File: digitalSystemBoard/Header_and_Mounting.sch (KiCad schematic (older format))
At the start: 16 parts, among them J10 Conn_02x03_Odd_Even, J11 Conn_02x03_Odd_Even, J12 Conn_02x03_Odd_Even, J3 Conn_02x04_Odd_Even, J4 Conn_02x04_Odd_Even, J5 Conn_02x08_Odd_Even, J6 Conn_02x07_Odd_Even, J7 Conn_02x07_Odd_Even, J8 Conn_02x08_Odd_Even, J9 Conn_02x03_Odd_Even

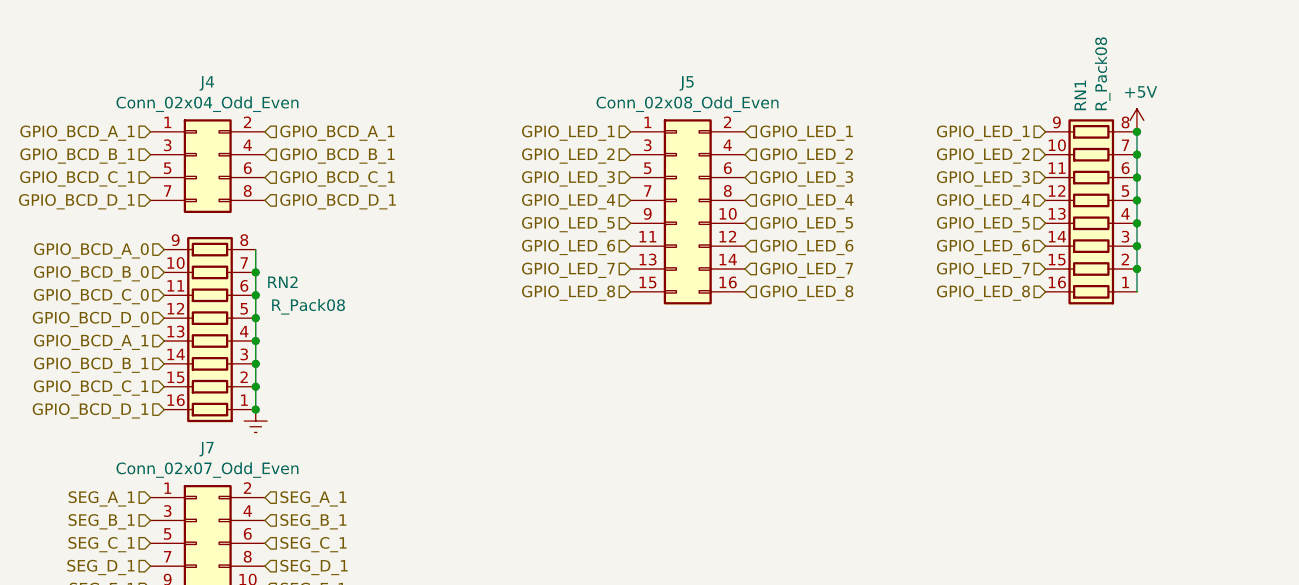
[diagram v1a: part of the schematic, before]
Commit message: Replace R array by 16 single R
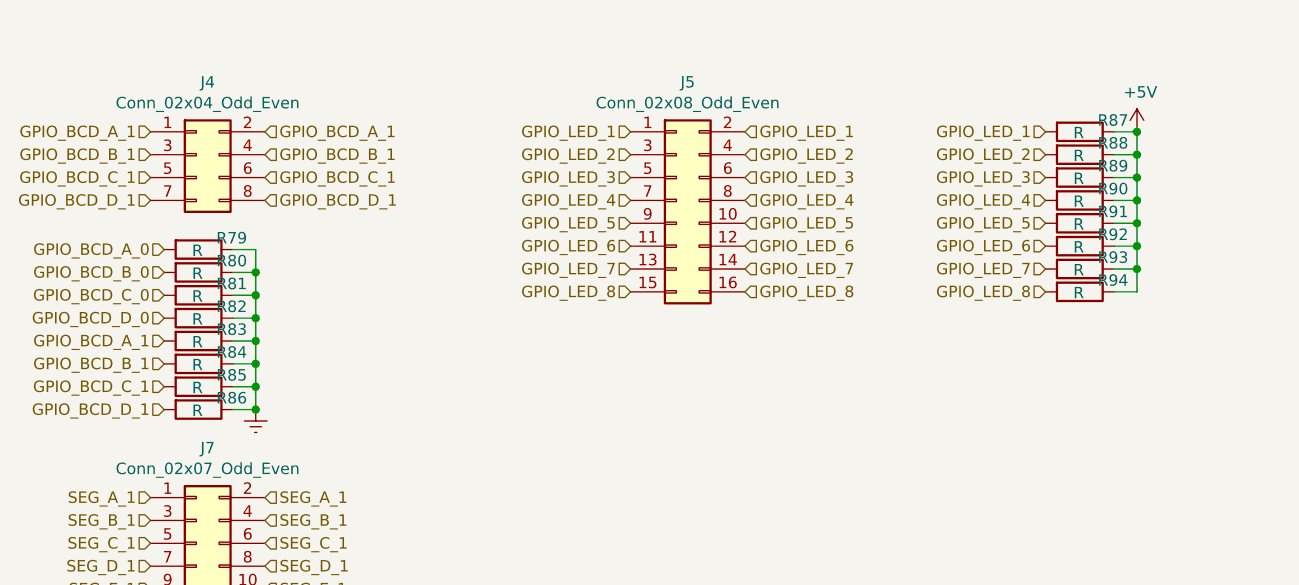
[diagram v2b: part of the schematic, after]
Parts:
- removed RN1, RN2: R_Pack08, digitalSystemBoard:Resistor Bar 06030 8P4R, symbol Device:R_Pack08
- added R79, R80, R81, R82, R83, R84, R85, R86, R87, R88, R89, R90, R91, R92, R93, R94: R, Resistor_SMD:R_0603_1608Metric, symbol Device:R
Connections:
- net +5V: now also R87.1, R88.1, R89.1, R90.1, R91.1, R92.1, R93.1, R94.1
- net Earth: now also R79.1, R80.1, R81.1, R82.1, R83.1, R84.1, R85.1, R86.1
- net GPIO_BCD_A_0: now also R79.2
- net GPIO_BCD_A_1: now also R83.2
- net GPIO_BCD_B_0: now also R80.2
- net GPIO_BCD_B_1: now also R84.2
- net GPIO_BCD_C_0: now also R81.2
- net GPIO_BCD_C_1: now also R85.2
- net GPIO_BCD_D_0: now also R82.2
- net GPIO_BCD_D_1: now also R86.2
- net GPIO_LED_1: now also R87.2
- net GPIO_LED_2: now also R88.2
- net GPIO_LED_3: now also R89.2
- net GPIO_LED_4: now also R90.2
- net GPIO_LED_5: now also R91.2
- net GPIO_LED_6: now also R92.2
- net GPIO_LED_7: now also R93.2
- net GPIO_LED_8: now also R94.2
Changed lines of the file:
@@
-$EndComp
-$Comp
-L Connector_Generic:Conn_02x04_Odd_Even J4
-U 1 1 5FC88FC0
-P 4000 2100
-F 0 "J4" H 4050 2417 50  0000 C CNN
-F 1 "Conn_02x04_Odd_Even" H 4050 2326 50  0000 C CNN
-F 2 "Connector_IDC:IDC-Header_2x04_P2.54mm_Vertical" H 4000 2100 50  0001 C CNN
-F 3 "~" H 4000 2100 50  0001 C CNN
-	1    4000 2100
-	1    0    0    -1
 $EndComp
 $Comp
@@
 SEG_A_1
 $Comp
-L Device:R_Pack08 RN1
-U 1 1 6033D84A
-P 7915 2300
-F 0 "RN1" H 8303 2346 50  0000 L CNN
-F 1 "R_Pack08" H 8303 2255 50  0000 L CNN
-F 2 "digitalSystemBoard:Resistor Bar 06030 8P4R" V 8390 2300 50  0001 C CNN
-F 3 "~" H 7915 2300 50  0001 C CNN
-	1    7915 2300
-	0    -1   -1   0
-$EndComp
-$Comp
-L Device:R_Pack08 RN2
-U 1 1 6033EE65
-P 4060 2815
-F 0 "RN2" V 4215 2425 50  0000 L CNN
-F 1 "R_Pack08" V 4115 2220 50  0000 L CNN
-F 2 "digitalSystemBoard:Resistor Bar 06030 8P4R" V 4535 2815 50  0001 C CNN
-F 3 "~" H 4060 2815 50  0001 C CNN
-	1    4060 2815
-	0    -1   -1   0
-$EndComp
-$Comp
 L power:+5V #PWR0101
 U 1 1 6049CAFD
@@
 	1    0    0    -1
 $EndComp
-Wire Wire Line
-	8115 2000 8115 2100
-Connection ~ 8115 2000
-Wire Wire Line
-	8115 2100 8115 2200
-Connection ~ 8115 2100
-Wire Wire Line
-	8115 2200 8115 2300
-Connection ~ 8115 2200
-Wire Wire Line
-	8115 2300 8115 2400
-Connection ~ 8115 2300
-Wire Wire Line
-	8115 2400 8115 2500
-Connection ~ 8115 2400
-Wire Wire Line
-	8115 2500 8115 2600
-Connection ~ 8115 2500
-Wire Wire Line
-	8115 2600 8115 2700
-Connection ~ 8115 2600
 Text HLabel 7715 2700 0    50   Input ~ 0
 GPIO_LED_8
@@
 Text HLabel 7715 2000 0    50   Input ~ 0
 GPIO_LED_1
-$Comp
-L power:Earth #PWR0102
-U 1 1 604ACAC7
-P 4260 3215
-F 0 "#PWR0102" H 4260 2965 50  0001 C CNN
-F 1 "Earth" H 4260 3065 50  0001 C CNN
-F 2 "" H 4260 3215 50  0001 C CNN
-F 3 "~" H 4260 3215 50  0001 C CNN
-	1    4260 3215
-	1    0    0    -1
-$EndComp
-Wire Wire Line
-	4260 2515 4260 2615
-Wire Wire Line
-	4260 2615 4260 2715
-Connection ~ 4260 2615
-Wire Wire Line
-	4260 2715 4260 2815
-Connection ~ 4260 2715
-Wire Wire Line
-	4260 2815 4260 2915
-Connection ~ 4260 2815
-Wire Wire Line
-	4260 2915 4260 3015
-Connection ~ 4260 2915
-Wire Wire Line
-	4260 3015 4260 3115
-Connection ~ 4260 3015
-Wire Wire Line
-	4260 3115 4260 3215
-Connection ~ 4260 3115
-Connection ~ 4260 3215
 Text HLabel 3860 2515 0    50   Input ~ 0
 GPIO_BCD_A_0
@@
 Text HLabel 3860 3215 0    50   Input ~ 0
 GPIO_BCD_D_1
+$Comp
+L Connector_Generic:Conn_02x04_Odd_Even J4
+U 1 1 5FC88FC0
+P 4000 2100
+F 0 "J4" H 4050 2417 50  0000 C CNN
+F 1 "Conn_02x04_Odd_Even" H 4050 2326 50  0000 C CNN
+F 2 "Connector_IDC:IDC-Header_2x04_P2.54mm_Vertical" H 4000 2100 50  0001 C CNN
+F 3 "~" H 4000 2100 50  0001 C CNN
+	1    4000 2100
+	1    0    0    -1
+$EndComp
+Connection ~ 4260 3215
+Wire Wire Line
+	4160 3215 4260 3215
+Wire Wire Line
+	4260 3115 4260 3215
+Connection ~ 4260 3115
+Wire Wire Line
+	4160 3115 4260 3115
+Wire Wire Line
+	4260 3015 4260 3115
+Connection ~ 4260 3015
+Wire Wire Line
+	4160 3015 4260 3015
+Wire Wire Line
+	4260 2915 4260 3015
+Connection ~ 4260 2915
+Wire Wire Line
+	4160 2915 4260 2915
+Wire Wire Line
+	4260 2815 4260 2915
+Connection ~ 4260 2815
+Wire Wire Line
+	4160 2815 4260 2815
+Wire Wire Line
+	4260 2715 4260 2815
+Connection ~ 4260 2715
+Wire Wire Line
+	4160 2715 4260 2715
+Wire Wire Line
+	4260 2615 4260 2715
+Connection ~ 4260 2615
+Wire Wire Line
+	4160 2615 4260 2615
+Wire Wire Line
+	4260 2515 4160 2515
+$Comp
+L Device:R R86
+U 1 1 60520B8F
+P 4010 3215
+F 0 "R86" V 3960 3360 50  0000 C CNN
+F 1 "R" V 4015 3210 50  0000 C CNN
+F 2 "Resistor_SMD:R_0603_1608Metric" V 3940 3215 50  0001 C CNN
+F 3 "~" H 4010 3215 50  0001 C CNN
+	1    4010 3215
+	0    1    1    0
+$EndComp
+$Comp
+L Device:R R85
+U 1 1 605206C3
+P 4010 3115
+F 0 "R85" V 3960 3260 50  0000 C CNN
+F 1 "R" V 4015 3110 50  0000 C CNN
+F 2 "Resistor_SMD:R_0603_1608Metric" V 3940 3115 50  0001 C CNN
+F 3 "~" H 4010 3115 50  0001 C CNN
+	1    4010 3115
+	0    1    1    0
+$EndComp
+$Comp
+L Device:R R84
+U 1 1 605202F2
+P 4010 3015
+F 0 "R84" V 3960 3160 50  0000 C CNN
+F 1 "R" V 4015 3010 50  0000 C CNN
+F 2 "Resistor_SMD:R_0603_1608Metric" V 3940 3015 50  0001 C CNN
+F 3 "~" H 4010 3015 50  0001 C CNN
+	1    4010 3015
+	0    1    1    0
+$EndComp
+$Comp
+L Device:R R83
+U 1 1 6051FA6A
+P 4010 2915
+F 0 "R83" V 3960 3060 50  0000 C CNN
+F 1 "R" V 4015 2910 50  0000 C CNN
+F 2 "Resistor_SMD:R_0603_1608Metric" V 3940 2915 50  0001 C CNN
+F 3 "~" H 4010 2915 50  0001 C CNN
+	1    4010 2915
+	0    1    1    0
+$EndComp
+$Comp
+L Device:R R82
+U 1 1 6051F3E2
+P 4010 2815
+F 0 "R82" V 3960 2960 50  0000 C CNN
+F 1 "R" V 4015 2810 50  0000 C CNN
+F 2 "Resistor_SMD:R_0603_1608Metric" V 3940 2815 50  0001 C CNN
+F 3 "~" H 4010 2815 50  0001 C CNN
+	1    4010 2815
+	0    1    1    0
+$EndComp
+$Comp
+L Device:R R81
+U 1 1 6051ECC9
+P 4010 2715
+F 0 "R81" V 3960 2860 50  0000 C CNN
+F 1 "R" V 4015 2710 50  0000 C CNN
+F 2 "Resistor_SMD:R_0603_1608Metric" V 3940 2715 50  0001 C CNN
+F 3 "~" H 4010 2715 50  0001 C CNN
+	1    4010 2715
+	0    1    1    0
+$EndComp
+$Comp
+L Device:R R80
+U 1 1 6051E775
+P 4010 2615
+F 0 "R80" V 3960 2760 50  0000 C CNN
+F 1 "R" V 4015 2610 50  0000 C CNN
+F 2 "Resistor_SMD:R_0603_1608Metric" V 3940 2615 50  0001 C CNN
+F 3 "~" H 4010 2615 50  0001 C CNN
+	1    4010 2615
+	0    1    1    0
+$EndComp
+$Comp
+L Device:R R79
+U 1 1 6051C220
+P 4010 2515
+F 0 "R79" V 3960 2660 50  0000 C CNN
+F 1 "R" V 4015 2510 50  0000 C CNN
+F 2 "Resistor_SMD:R_0603_1608Metric" V 3940 2515 50  0001 C CNN
+F 3 "~" H 4010 2515 50  0001 C CNN
+	1    4010 2515
+	0    1    1    0
+$EndComp
+Wire Wire Line
+	4260 2515 4260 2615
+$Comp
+L power:Earth #PWR0102
+U 1 1 604ACAC7
+P 4260 3215
+F 0 "#PWR0102" H 4260 2965 50  0001 C CNN
+F 1 "Earth" H 4260 3065 50  0001 C CNN
+F 2 "" H 4260 3215 50  0001 C CNN
+F 3 "~" H 4260 3215 50  0001 C CNN
+	1    4260 3215
+	1    0    0    -1
+$EndComp
+Wire Wire Line
+	8015 2700 8115 2700
+Wire Wire Line
+	8115 2600 8115 2700
+Connection ~ 8115 2600
+Wire Wire Line
+	8015 2600 8115 2600
+Wire Wire Line
+	8115 2500 8115 2600
+Connection ~ 8115 2500
+Wire Wire Line
+	8015 2500 8115 2500
+Wire Wire Line
+	8115 2400 8115 2500
+Connection ~ 8115 2400
+Wire Wire Line
+	8015 2400 8115 2400
+Wire Wire Line
+	8115 2300 8115 2400
+Connection ~ 8115 2300
+Wire Wire Line
+	8015 2300 8115 2300
+Wire Wire Line
+	8115 2200 8115 2300
+Connection ~ 8115 2200
+Wire Wire Line
+	8015 2200 8115 2200
+Wire Wire Line
+	8115 2100 8115 2200
+Connection ~ 8115 2100
+Wire Wire Line
+	8015 2100 8115 2100
+Wire Wire Line
+	8115 2000 8015 2000
+$Comp
+L Device:R R94
+U 1 1 6052A04C
+P 7865 2700
+F 0 "R94" V 7815 2845 50  0000 C CNN
+F 1 "R" V 7870 2695 50  0000 C CNN
+F 2 "Resistor_SMD:R_0603_1608Metric" V 7795 2700 50  0001 C CNN
+F 3 "~" H 7865 2700 50  0001 C CNN
+	1    7865 2700
+	0    1    1    0
+$EndComp
+$Comp
+L Device:R R93
+U 1 1 6052A056
+P 7865 2600
+F 0 "R93" V 7815 2745 50  0000 C CNN
+F 1 "R" V 7870 2595 50  0000 C CNN
+F 2 "Resistor_SMD:R_0603_1608Metric" V 7795 2600 50  0001 C CNN
+F 3 "~" H 7865 2600 50  0001 C CNN
+	1    7865 2600
+	0    1    1    0
+$EndComp
+$Comp
+L Device:R R92
+U 1 1 6052A060
+P 7865 2500
+F 0 "R92" V 7815 2645 50  0000 C CNN
+F 1 "R" V 7870 2495 50  0000 C CNN
+F 2 "Resistor_SMD:R_0603_1608Metric" V 7795 2500 50  0001 C CNN
+F 3 "~" H 7865 2500 50  0001 C CNN
+	1    7865 2500
+	0    1    1    0
+$EndComp
+$Comp
+L Device:R R91
+U 1 1 6052A06A
+P 7865 2400
+F 0 "R91" V 7815 2545 50  0000 C CNN
+F 1 "R" V 7870 2395 50  0000 C CNN
+F 2 "Resistor_SMD:R_0603_1608Metric" V 7795 2400 50  0001 C CNN
+F 3 "~" H 7865 2400 50  0001 C CNN
+	1    7865 2400
+	0    1    1    0
+$EndComp
+$Comp
+L Device:R R90
+U 1 1 6052A074
+P 7865 2300
+F 0 "R90" V 7815 2445 50  0000 C CNN
+F 1 "R" V 7870 2295 50  0000 C CNN
+F 2 "Resistor_SMD:R_0603_1608Metric" V 7795 2300 50  0001 C CNN
+F 3 "~" H 7865 2300 50  0001 C CNN
+	1    7865 2300
+	0    1    1    0
+$EndComp
+$Comp
+L Device:R R89
+U 1 1 6052A07E
+P 7865 2200
+F 0 "R89" V 7815 2345 50  0000 C CNN
+F 1 "R" V 7870 2195 50  0000 C CNN
+F 2 "Resistor_SMD:R_0603_1608Metric" V 7795 2200 50  0001 C CNN
+F 3 "~" H 7865 2200 50  0001 C CNN
+	1    7865 2200
+	0    1    1    0
+$EndComp
+$Comp
+L Device:R R88
+U 1 1 6052A088
+P 7865 2100
+F 0 "R88" V 7815 2245 50  0000 C CNN
+F 1 "R" V 7870 2095 50  0000 C CNN
+F 2 "Resistor_SMD:R_0603_1608Metric" V 7795 2100 50  0001 C CNN
+F 3 "~" H 7865 2100 50  0001 C CNN
+	1    7865 2100
+	0    1    1    0
+$EndComp
+$Comp
+L Device:R R87
+U 1 1 6052A092
+P 7865 2000
+F 0 "R87" V 7815 2145 50  0000 C CNN
+F 1 "R" V 7870 1995 50  0000 C CNN
+F 2 "Resistor_SMD:R_0603_1608Metric" V 7795 2000 50  0001 C CNN
+F 3 "~" H 7865 2000 50  0001 C CNN
+	1    7865 2000
+	0    1    1    0
+$EndComp
+Wire Wire Line
+	8115 2000 8115 2100
+Connection ~ 8115 2000
 $EndSCHEMATC

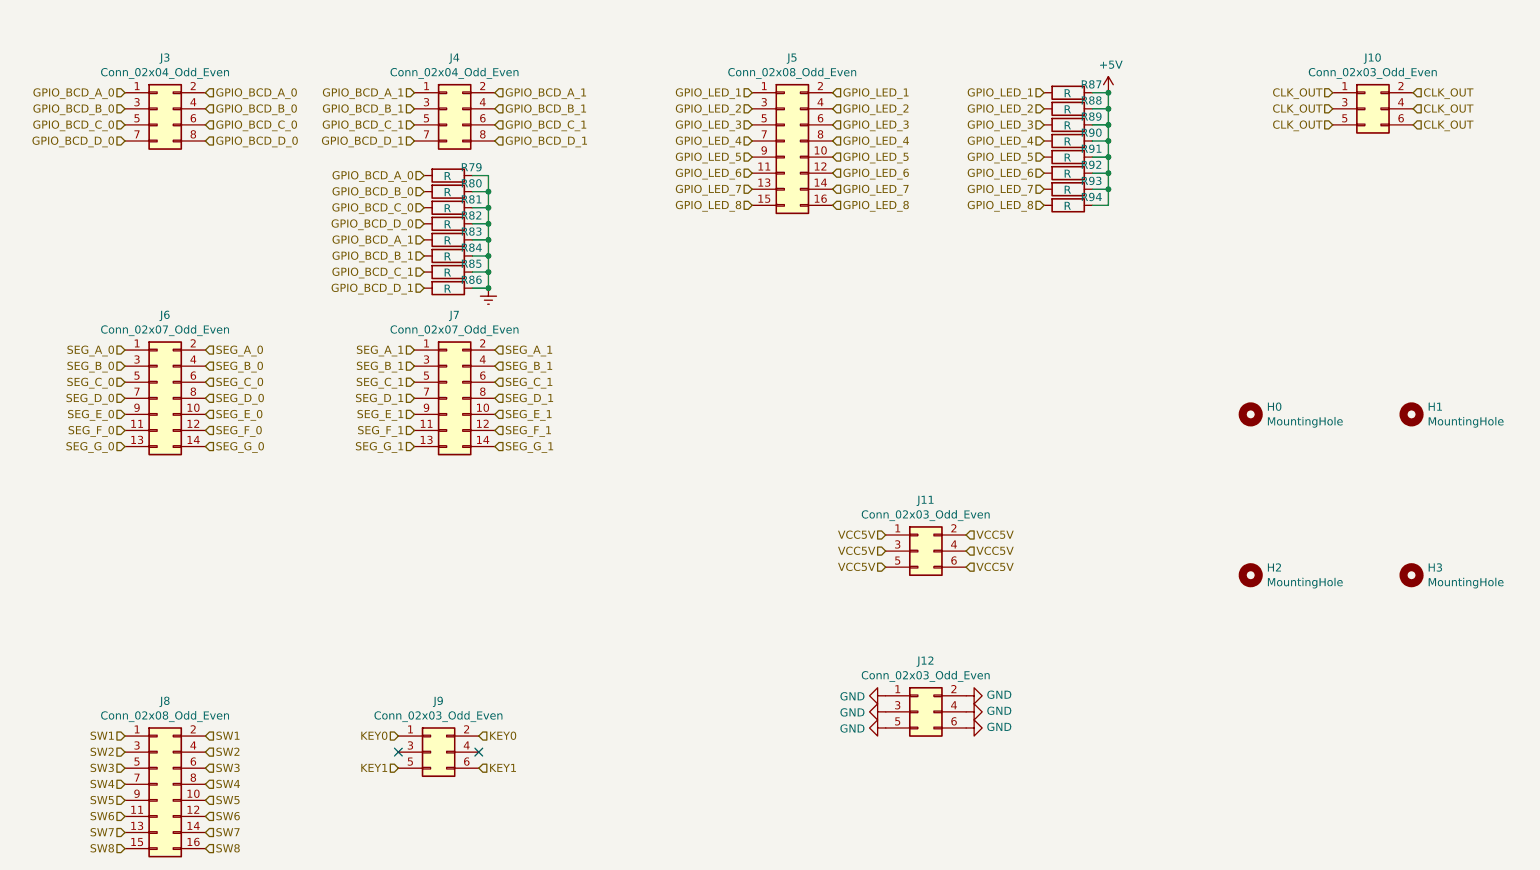
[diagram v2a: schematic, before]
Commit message: Add IC 74HC595 and R for input pin
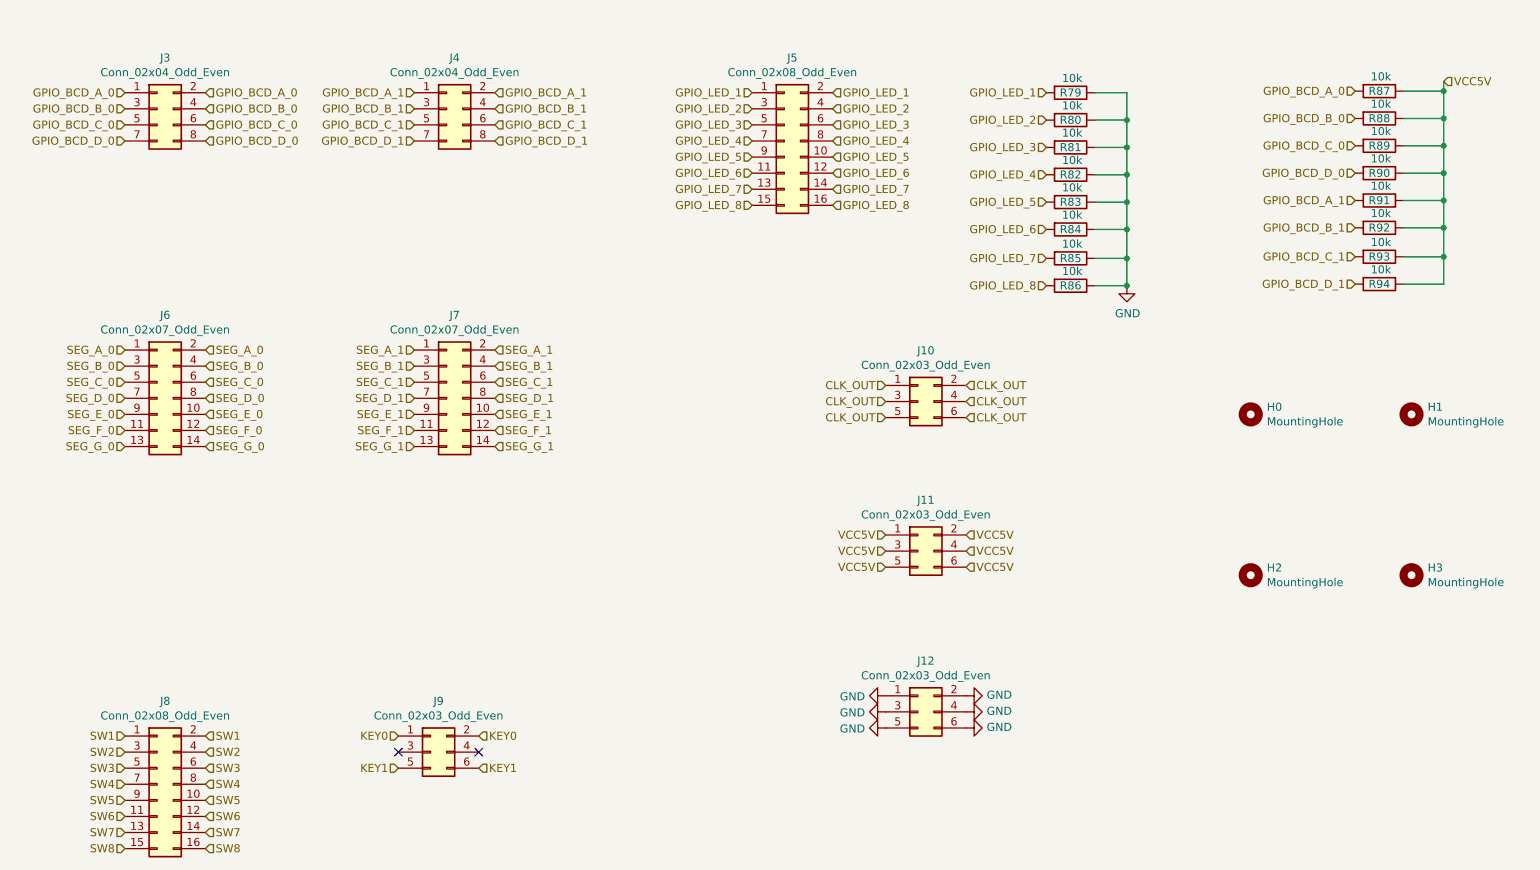
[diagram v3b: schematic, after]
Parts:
- R79, R80, R81, R82, R83, R84, R85, R86, R87, R88, R89, R90, R91, R92, R93, R94: value R -> 10k
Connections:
- net +5V is gone; now on net VCC5V: R87.1, R88.1, R89.1, R90.1, R91.1, R92.1, R93.1, R94.1
- net Earth is gone; now on net GND: R79.1, R80.1, R81.1, R82.1, R83.1, R84.1, R85.1, R86.1
- net GPIO_BCD_A_0: now also R87.2; no longer R79.2
- net GPIO_BCD_A_1: now also R91.2; no longer R83.2
- net GPIO_BCD_B_0: now also R88.2; no longer R80.2
- net GPIO_BCD_B_1: now also R92.2; no longer R84.2
- net GPIO_BCD_C_0: now also R89.2; no longer R81.2
- net GPIO_BCD_C_1: now also R93.2; no longer R85.2
- net GPIO_BCD_D_0: now also R90.2; no longer R82.2
- net GPIO_BCD_D_1: now also R94.2; no longer R86.2
- net GPIO_LED_1: now also R79.2; no longer R87.2
- net GPIO_LED_2: now also R80.2; no longer R88.2
- net GPIO_LED_3: now also R81.2; no longer R89.2
- net GPIO_LED_4: now also R82.2; no longer R90.2
- net GPIO_LED_5: now also R83.2; no longer R91.2
- net GPIO_LED_6: now also R84.2; no longer R92.2
- net GPIO_LED_7: now also R85.2; no longer R93.2
- net GPIO_LED_8: now also R86.2; no longer R94.2
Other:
- moved on the sheet: J10
